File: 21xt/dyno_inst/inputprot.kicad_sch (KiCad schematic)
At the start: 23 parts, among them U1 1SS362FV_L3F, U10 ADA4945-1ACPZ-R2, U2 1SS362FV_L3F, U4 1SS362FV_L3F, U9 1SS362FV_L3F

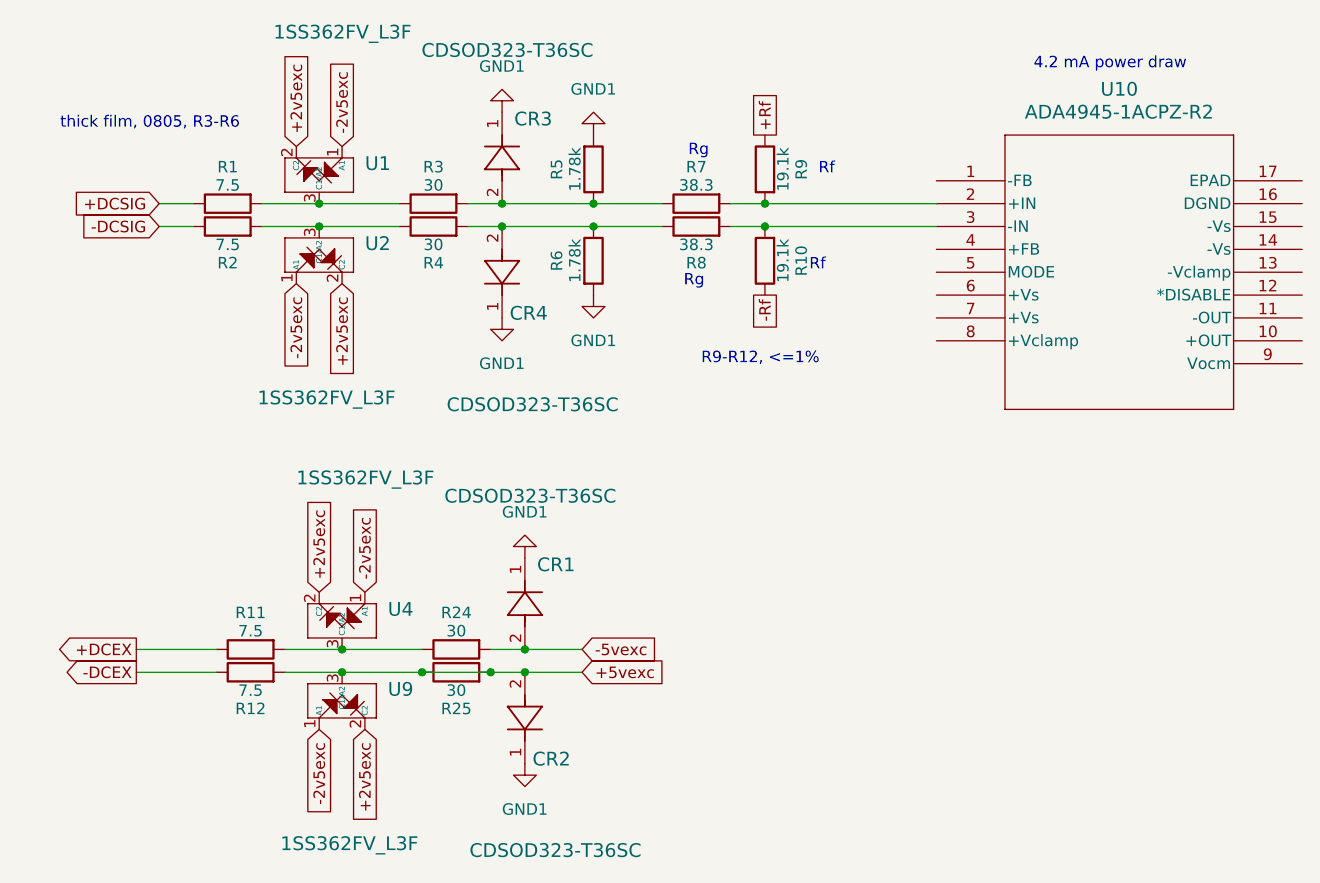
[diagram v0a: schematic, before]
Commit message: ye
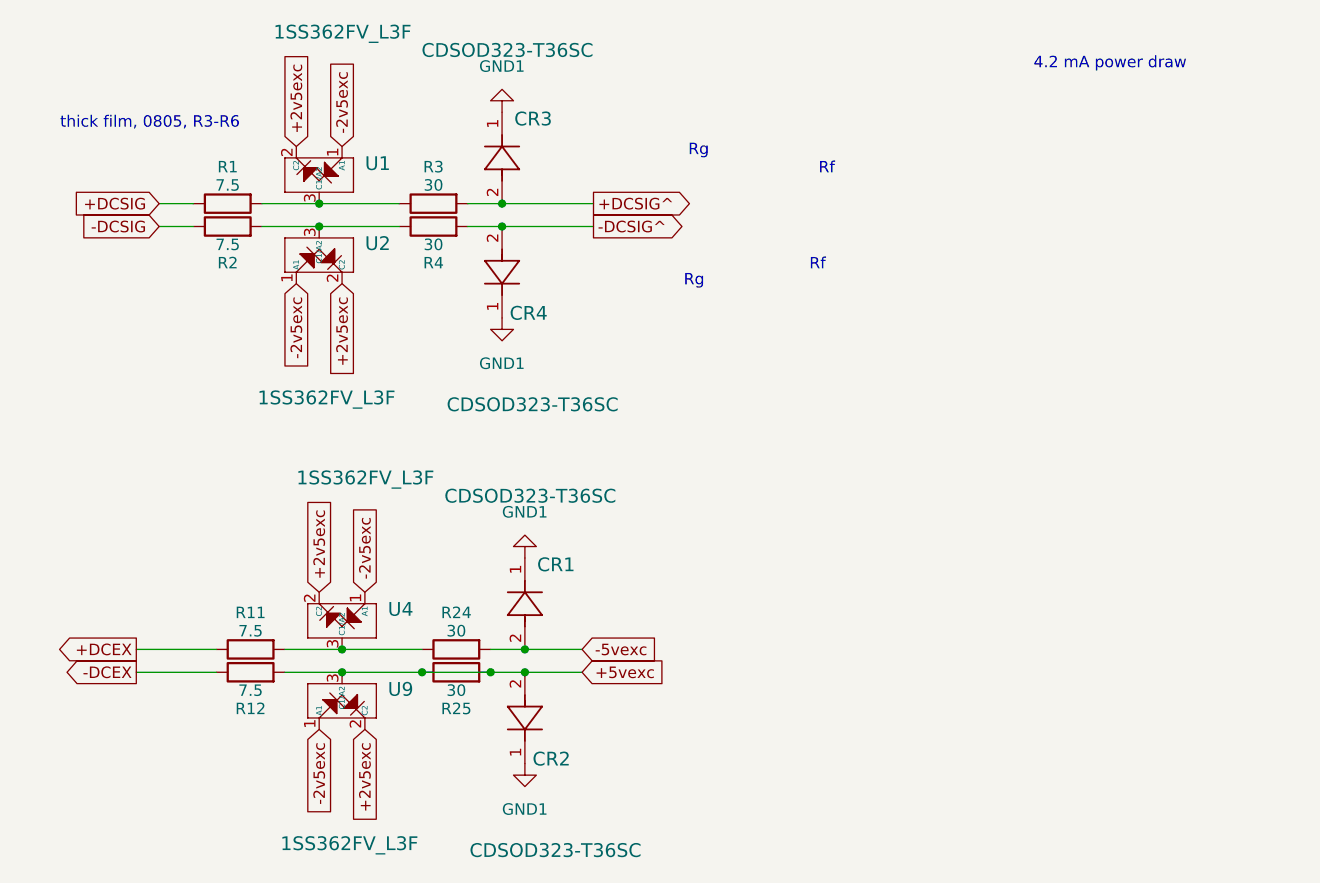
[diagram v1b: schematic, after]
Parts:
- removed R10, R9: 19.1k, symbol Device:R
- removed R5, R6: 1.78k, symbol Device:R
- removed R7, R8: 38.3, symbol Device:R
- removed U10: ADA4945-1ACPZ-R2, LFCSP16_ADA4945-1ACPZ-R2_ADI, symbol dyno_inst_sym:ADA4945-1ACPZ-R2
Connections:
- net -DCSIG^: now reaches CR4.2, R4.2
- net +DCSIG^: now reaches CR3.2, R3.2
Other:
- note removed: "R9-R12, <=1%"
